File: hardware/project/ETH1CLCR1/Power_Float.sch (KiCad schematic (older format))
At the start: 56 parts, among them U602 LM1117IMP-3.3/NOPB, U604 LM1117IMP-3.3/NOPB, U608 LM1117IMP-5.0/NOPB, U609 TSR1-2490, U701 THL15-2415WI, U705 TSR2-2450, U706 LT8330_S6, U710 LT8330_S6

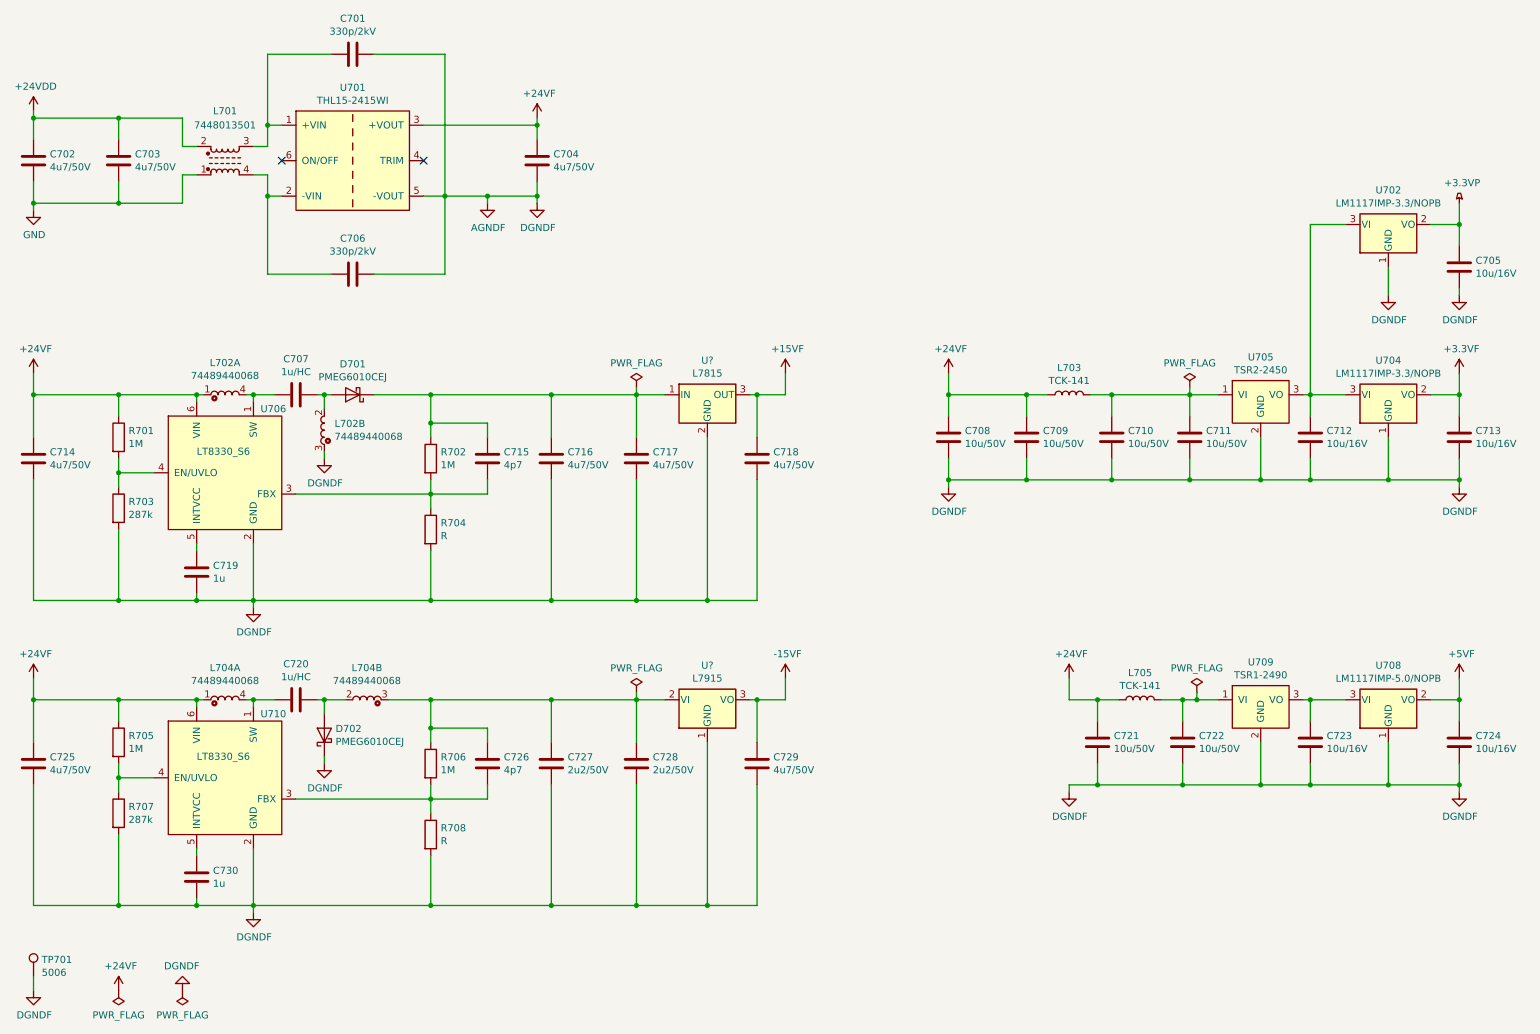
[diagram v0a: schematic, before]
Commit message: Schematic design
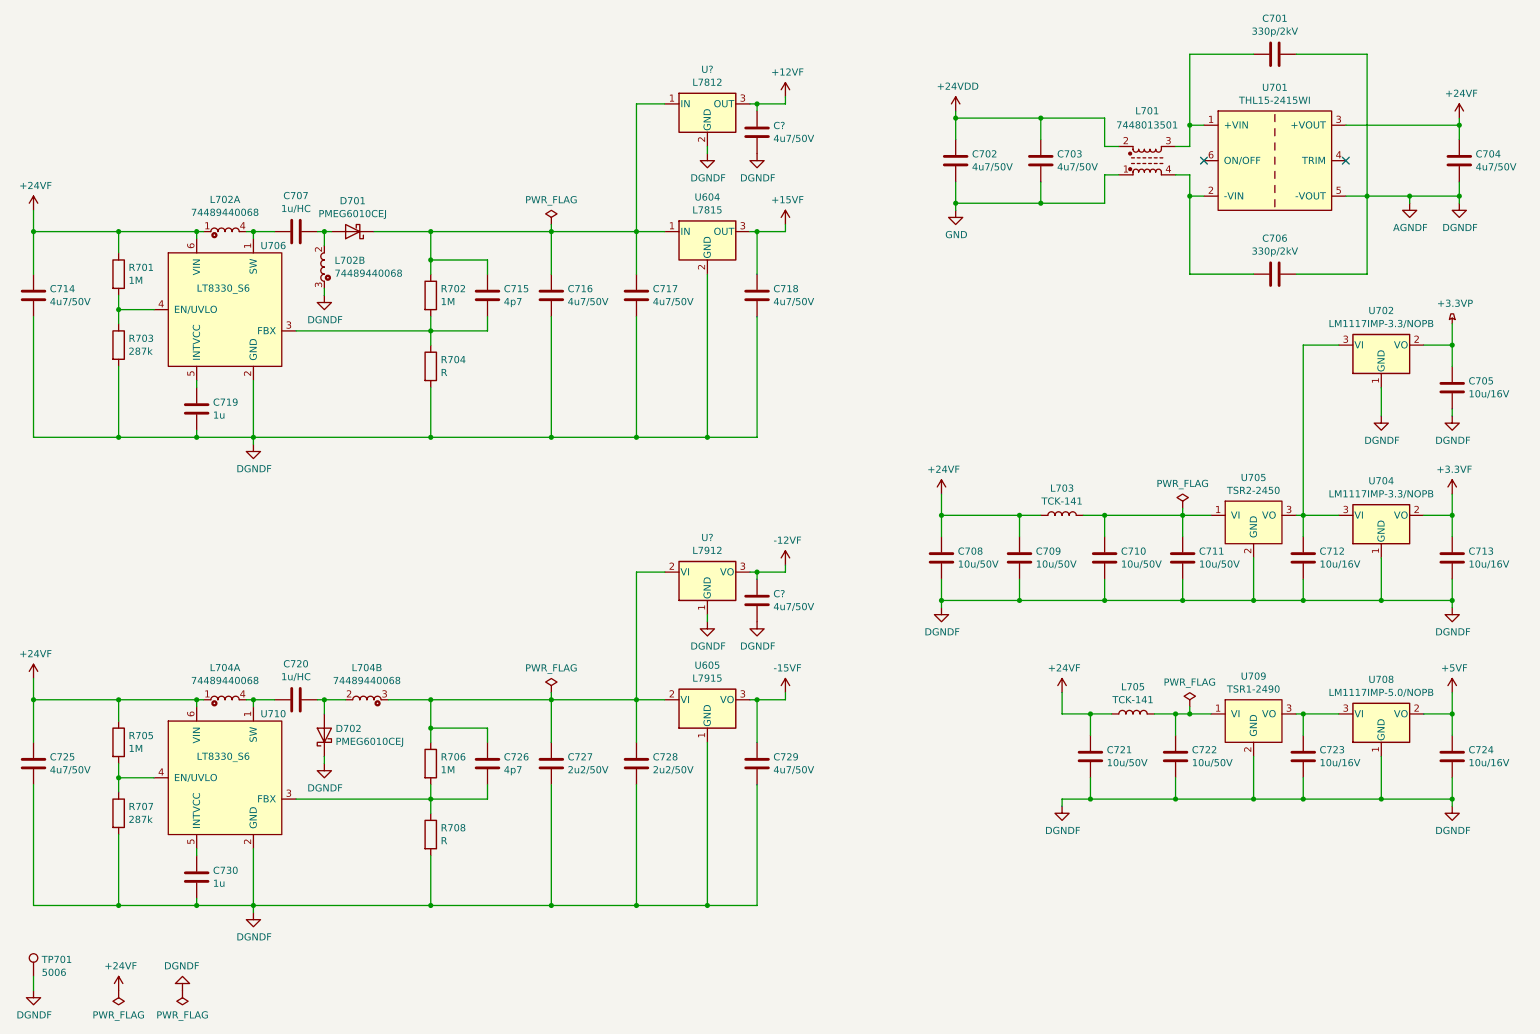
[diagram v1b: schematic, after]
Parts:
- added C? (x2): 4u7/50V, Capacitor_SMD:C_1206_3216Metric_Pad1.42x1.75mm_HandSolder, symbol Device:C
- added U?: L7812, symbol Regulator_Linear:L7815
- added U?: L7912, symbol Regulator_Linear:L7915
- gave numbers to parts that had none: 2
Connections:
- net AGNDF: now also C?.2, C?.2, U?.1 (GND), U?.2 (GND)
- net at C715.1, C716.1, C717.1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: now also U?.1 (IN)
- net at C726.1, C727.1, C728.1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: now also U?.2 (VI)
- new net +12VF: C?.1, U?.3 (OUT)
- new net -12VF: C?.1, U?.3 (VO)
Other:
- moved on the sheet: C701, C702, C703, C704, C705, C706, C707, C708, C709, C710, C711, C712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
